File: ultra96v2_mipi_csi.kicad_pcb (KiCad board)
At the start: 2 copper layers, 85 x 54 mm, 42 parts, among them J1 61083-063402LF, J2 10075024-G01-20ULF, J3 1-1734248-5, J4 1-1734248-5, U1 AP7361C-33E, U2 SN74AVC4T245PW, U3 PCA9306, U4 PCA9306

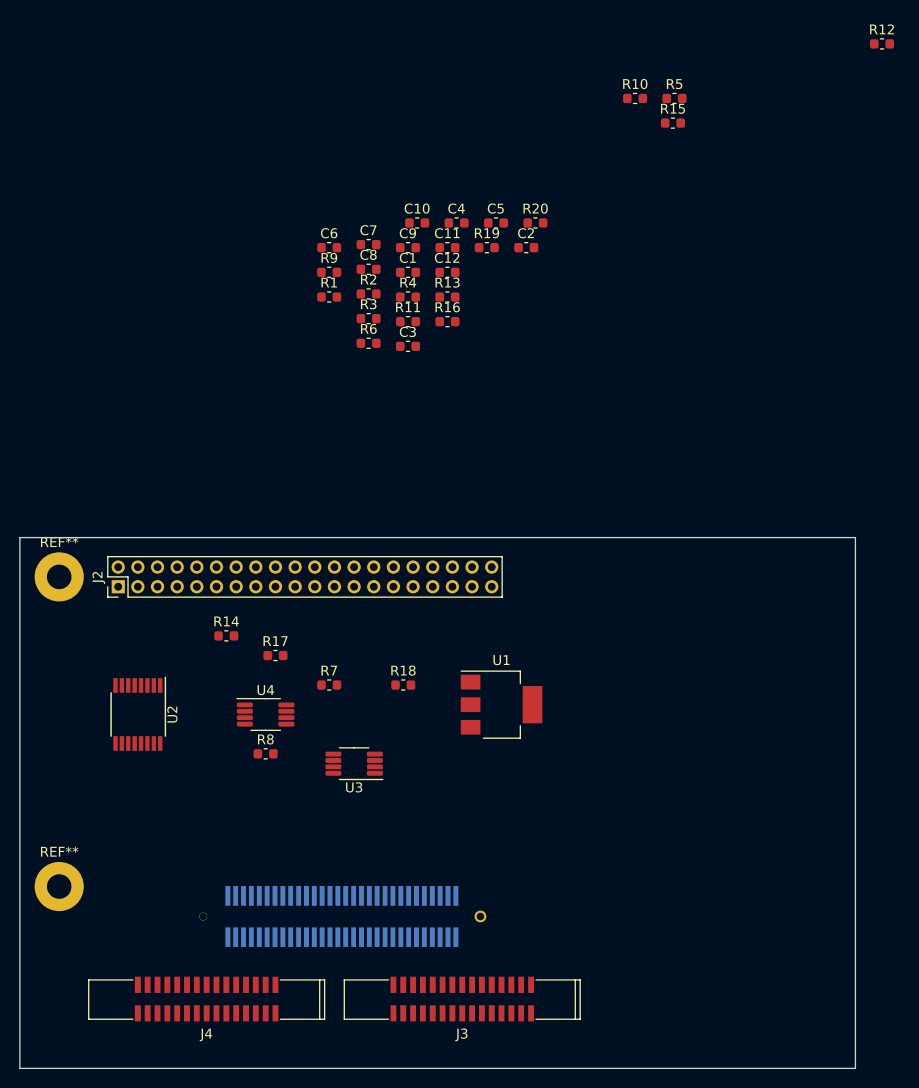
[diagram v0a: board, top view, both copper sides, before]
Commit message: update
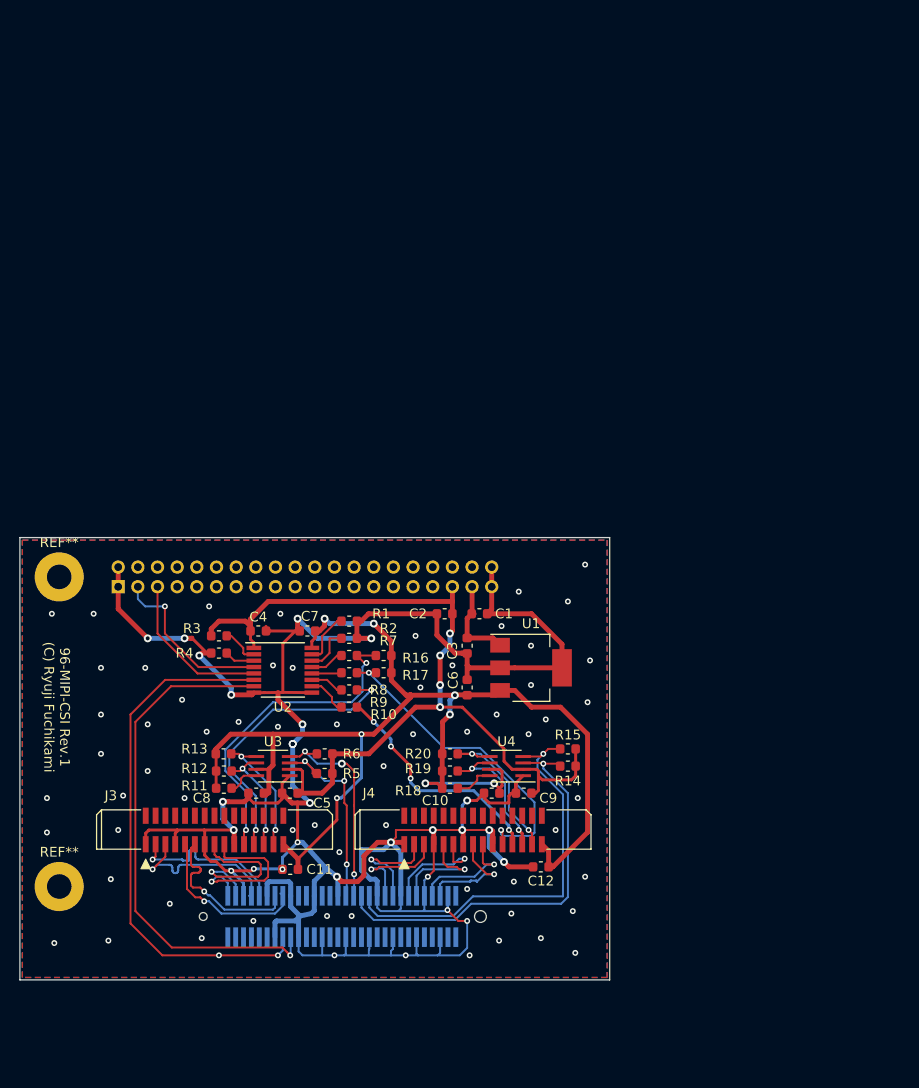
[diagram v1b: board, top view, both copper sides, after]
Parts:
- J2: footprint Connector_PinHeader_2.00mm:PinHeader_2x20_P2.00mm_Vertical -> Connector_PinSocket_2.00mm:PinSocket_2x20_P2.00mm_Vertical; moved to B.Cu
- U3, U4: value PCA9306 -> PCA9306DCTR; footprint Package_SO:MSOP-8_3x3mm_P0.65mm -> myfootprint:PCA9306DCTR
- moved R12 99.8 mm to (120.8, 123.8)
- moved R5 77.4 mm to (131.0, 124.0)
- moved R10 68.4 mm to (133.5, 117.2), turned to 180 degrees
- moved C11 65.2 mm to (127.5, 133.8), turned to 180 degrees
- moved R15 64.6 mm to (155.8, 121.5)
- moved C5 61.7 mm to (127.5, 126.0), turned to 180 degrees
- moved C12 61.2 mm to (153.0, 133.5), turned to 180 degrees
- moved C10 58.5 mm to (148.0, 126.0), turned to 180 degrees
- moved C9 56.7 mm to (151.2, 126.0), turned to 180 degrees
- moved R20 54.7 mm to (143.8, 122.0)
- moved C8 54.5 mm to (124.0, 126.0), turned to 180 degrees
- moved R19 53.4 mm to (143.8, 123.8)
- moved R13 51.8 mm to (120.7, 122.0)
- moved R11 51.0 mm to (120.8, 125.5)
- moved C6 46.9 mm to (145.5, 115.2), turned to 90 degrees
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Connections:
- J1 pad 56: Net-(J1-Pad56) -> /HS_CSI1_CLK_N
- J3 pad 5: /HS_CSI0_D1_P -> /HS_CSI0_D1_N
- J4 pad 5: /HS_CSI1_D1_P -> /HS_CSI1_D1_N
- U1 pad 2: Net-(U1-Pad2) -> GND
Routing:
- net GND: track 0.00 -> 306.9 mm, vias 0 -> 90
- net +3V3: track 0.00 -> 132.9 mm, vias 0 -> 8
- net +1V8: track 0.00 -> 92.0 mm, vias 0 -> 4
- net /HS_CSI0_MCLK: track 0.00 -> 53.7 mm, vias 0 -> 2
- net /HS_CSI1_MCLK: track 0.00 -> 52.3 mm, vias 0 -> 1
- net /HS_I2C3_SCL: track 0.00 -> 42.2 mm, vias 0 -> 1
- net /HS_I2C3_SDA: track 0.00 -> 42.0 mm, vias 0 -> 1
- net /CAM0_GPIO: track 0.00 -> 33.2 mm, vias 0 -> 2
- net /CAM1_GPIO: track 0.00 -> 32.9 mm, vias 0 -> 2
- net /CAM0_CLK: track 0.00 -> 29.0 mm, vias 0 -> 2
- net /CAM1_CLK: track 0.00 -> 23.9 mm, vias 0 -> 4
- net /HS_I2C2_SDA: track 0.00 -> 22.2 mm, vias 0 -> 3
- net /HS_I2C2_SCL: track 0.00 -> 20.4 mm, vias 0 -> 3
- net /LS_GPIO_0: track 0.00 -> 17.5 mm, vias 0 -> 1
- net /HS_CSI0_D1_N: track 0.00 -> 17.1 mm, vias 0 -> 1
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- added copper zone on B.Cu, net GND
- added copper zone on F.Cu, net GND
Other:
- board size 85 x 54 mm -> 60 x 45 mm
- board text added: "96-MIPI-CSI Rev.1 (C) Ryuji Fuchikami"
